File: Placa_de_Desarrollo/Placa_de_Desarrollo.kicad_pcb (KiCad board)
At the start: 2 copper layers, 123.8 x 104.8 mm, 27 parts, among them J1 USB_B_Micro, J2 Conn_01x20, J3 ADC0, J4 ADC1, J5 ADC2, J6 Conn_01x14, SW1 RESET, U1 LM317_TO-220, U2 Pico

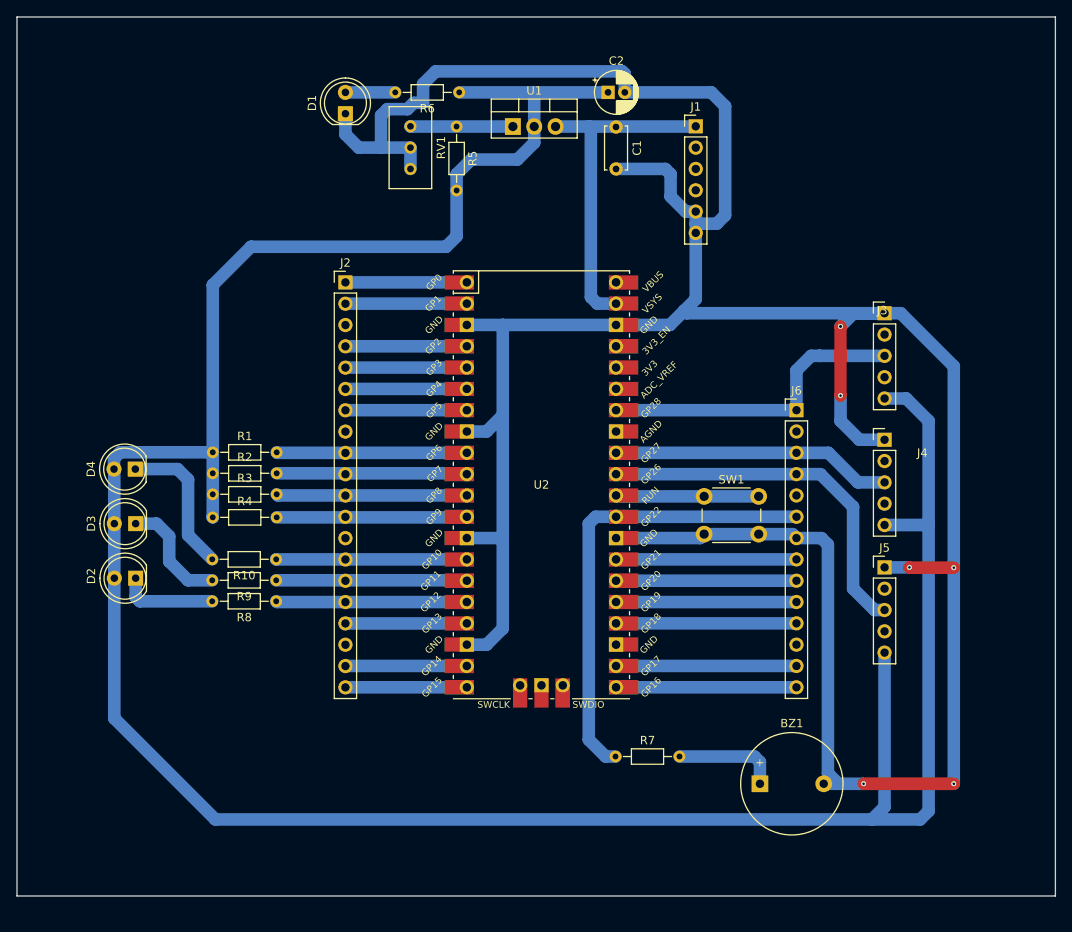
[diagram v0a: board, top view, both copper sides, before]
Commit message: Mejora de Placa de desarrollo
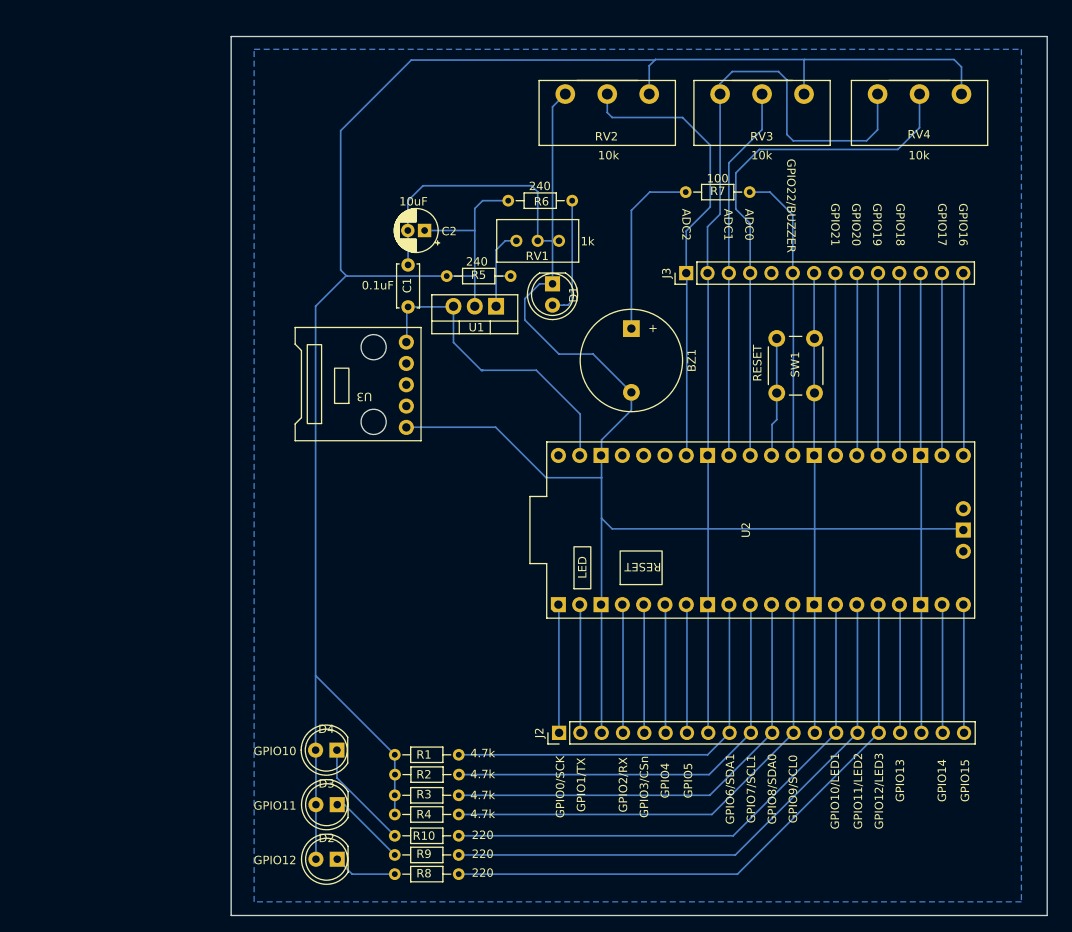
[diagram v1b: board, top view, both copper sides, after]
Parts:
- removed J1: USB_B_Micro, Connector_PinHeader_2.54mm:PinHeader_1x06_P2.54mm_Vertical
- removed the J3 at (186.9, 69.6)
- removed J4: ADC1, Connector_PinHeader_2.54mm:PinHeader_1x05_P2.54mm_Vertical
- removed J5: ADC2, Connector_PinHeader_2.54mm:PinHeader_1x05_P2.54mm_Vertical
- added RV2: 10k, Potentiometer_THT:Potentiometer_Piher_T-16H_Single_Horizontal, F.Cu at (158.8, 43.4)
- added RV3: 10k, Potentiometer_THT:Potentiometer_Piher_T-16H_Single_Horizontal, F.Cu at (177.3, 43.4)
- added RV4: 10k, Potentiometer_THT:Potentiometer_Piher_T-16H_Single_Horizontal, F.Cu at (196.1, 43.4)
- added U3: ~, Micro_USB_PCB:Micro_USB_B, F.Cu at (124.9, 79.0)
- SW1: footprint Button_Switch_THT:SW_PUSH_6mm_H9.5mm -> Button_Switch_THT:SW_PUSH_6mm
- U2: value Pico -> RP2350; footprint MCU_RaspberryPi_and_Boards:RPi_Pico_SMD_TH -> BoardF_Pi_Pico:BoardF_Pi_Pico_RP2350
- moved R7 69.1 mm to (170.8, 55.1), turned to 180 degrees
- moved J2 59.4 mm to (148.1, 119.6), turned to 90 degrees
- moved BZ1 56.4 mm to (156.7, 71.4), turned to -90 degrees
- moved R1 42.1 mm to (128.5, 122.2)
- moved R2 42.0 mm to (128.5, 124.5)
- moved R3 41.9 mm to (128.5, 127.0)
- moved R4 41.5 mm to (128.5, 129.3)
- moved D4 41.2 mm to (121.6, 121.6)
- moved D2 41.2 mm to (121.7, 134.6)
- moved D3 41.2 mm to (121.7, 128.1)
- moved R10 39.5 mm to (136.1, 131.8)
- moved R9 39.3 mm to (136.1, 134.1)
- moved R8 39.1 mm to (136.1, 136.4)
- moved C1 32.8 mm to (130.1, 68.8), turned to 90 degrees
- moved D1 31.9 mm to (147.3, 66.0), turned to -90 degrees
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- renumbered J6 to J3
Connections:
- J2 pad 13: unconnected-(J2-Pin_13-Pad13) -> GND
- J2 pad 18: unconnected-(J2-Pin_18-Pad18) -> GND
- J2 pad 3: unconnected-(J2-Pin_3-Pad3) -> GND
- J2 pad 8: unconnected-(J2-Pin_8-Pad8) -> GND
- J3 pad 12: unconnected-(J6-Pin_12-Pad12) -> GND
- J3 pad 2: unconnected-(J6-Pin_2-Pad2) -> GND
- U2 pad 33: unconnected-(U2-AGND-Pad33)_0 -> GND
- U2 pad 42: unconnected-(U2-GND-Pad42) -> GND
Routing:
- net 3.3V: track 325.3 -> 236.1 mm
- net LED3: track 22.8 -> 72.5 mm
- net LED2: track 22.7 -> 69.0 mm
- net LED1: track 22.7 -> 65.5 mm
- net GND: track 371.3 -> 409.2 mm, vias 7 -> 0
- net SCL0: track 22.7 -> 59.4 mm
- net SDA0: track 22.7 -> 55.9 mm
- net SCL1: track 22.7 -> 52.3 mm
- net SDA1: track 22.7 -> 48.9 mm
- net BUZZER: track 54.9 -> 34.9 mm
- net ADC0: track 44.4 -> 62.4 mm
- net ADC2: track 37.5 -> 54.1 mm
- net ADC1: track 33.5 -> 44.6 mm
- net Net-(BZ1-+): track 12.5 -> 21.5 mm
- net Net-(D1-A): track 5.94 -> 14.5 mm
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- added copper zone on B.Cu, net GND
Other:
- board size 123.8 x 104.8 mm -> 97.2 x 104.8 mm
- board text added: "0.1uF"
- board text added: "100"
- board text added: "10k"
- board text added: "10uF"
- board text added: "1k"
- board text added: "220"
- board text added: "240"
- board text added: "4.7k"
- board text added: "ADC0"
- board text added: "ADC1"
- board text added: "ADC2"
- board text added: "GPIO0/SCK"
- board text added: "GPIO1/TX"
- board text added: "GPIO10"
- board text added: "GPIO10/LED1"
- board text added: "GPIO11"
- board text added: "GPIO11/LED2"
- board text added: "GPIO12"
- board text added: "GPIO12/LED3"
- board text added: "GPIO13"
- board text added: "GPIO14"
- board text added: "GPIO15"
- board text added: "GPIO16"
- board text added: "GPIO17"
- board text added: "GPIO18"
- board text added: "GPIO19"
- board text added: "GPIO2/RX"
- board text added: "GPIO20"
- board text added: "GPIO21"
- board text added: "GPIO22/BUZZER"
- board text added: "GPIO3/CSn"
- board text added: "GPIO4"
- board text added: "GPIO5"
- board text added: "GPIO6/SDA1"
- board text added: "GPIO7/SCL1"
- board text added: "GPIO8/SDA0"
- board text added: "GPIO9/SCL0"
- board text added: "RESET"
